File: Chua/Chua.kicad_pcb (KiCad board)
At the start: 2 copper layers, 60 x 30 mm, 19 parts, among them P1 CONN_01X03, U1 TL082, U2 TL082

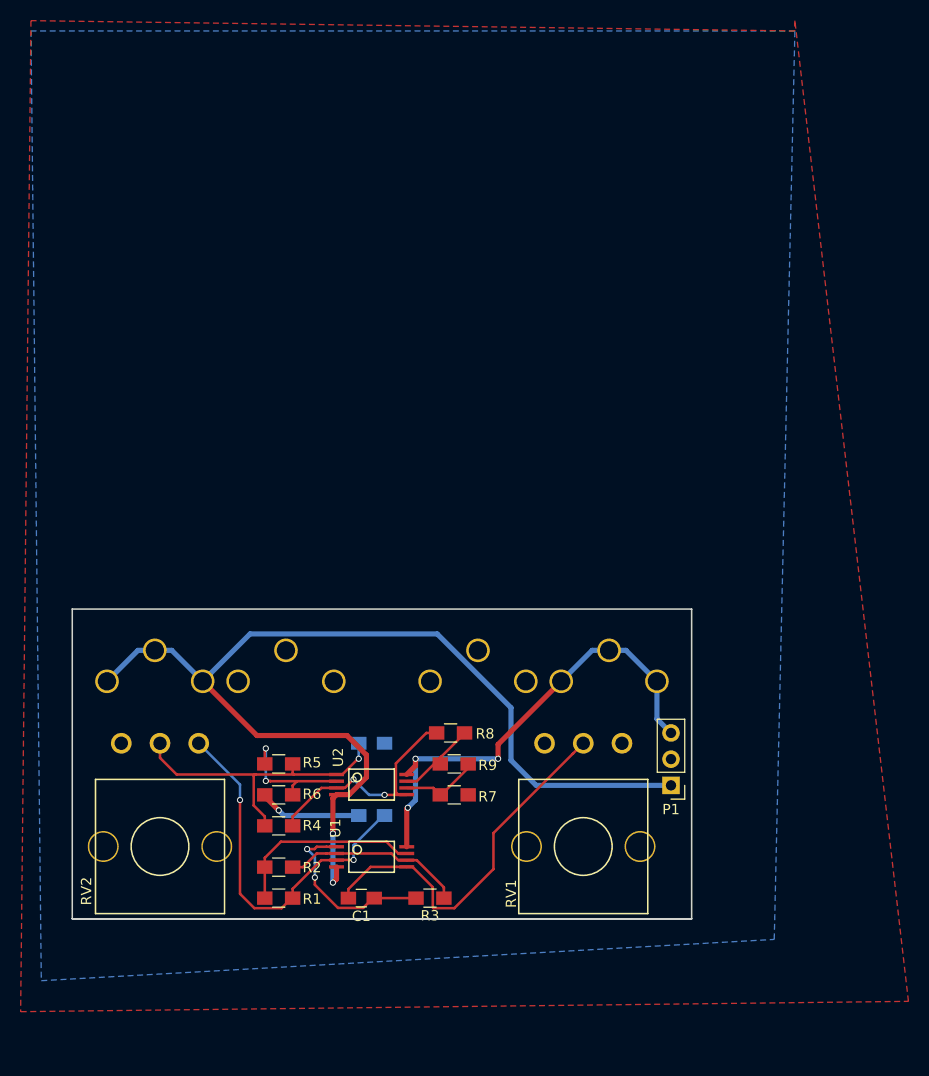
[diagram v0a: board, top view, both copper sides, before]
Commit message: adding output to chua
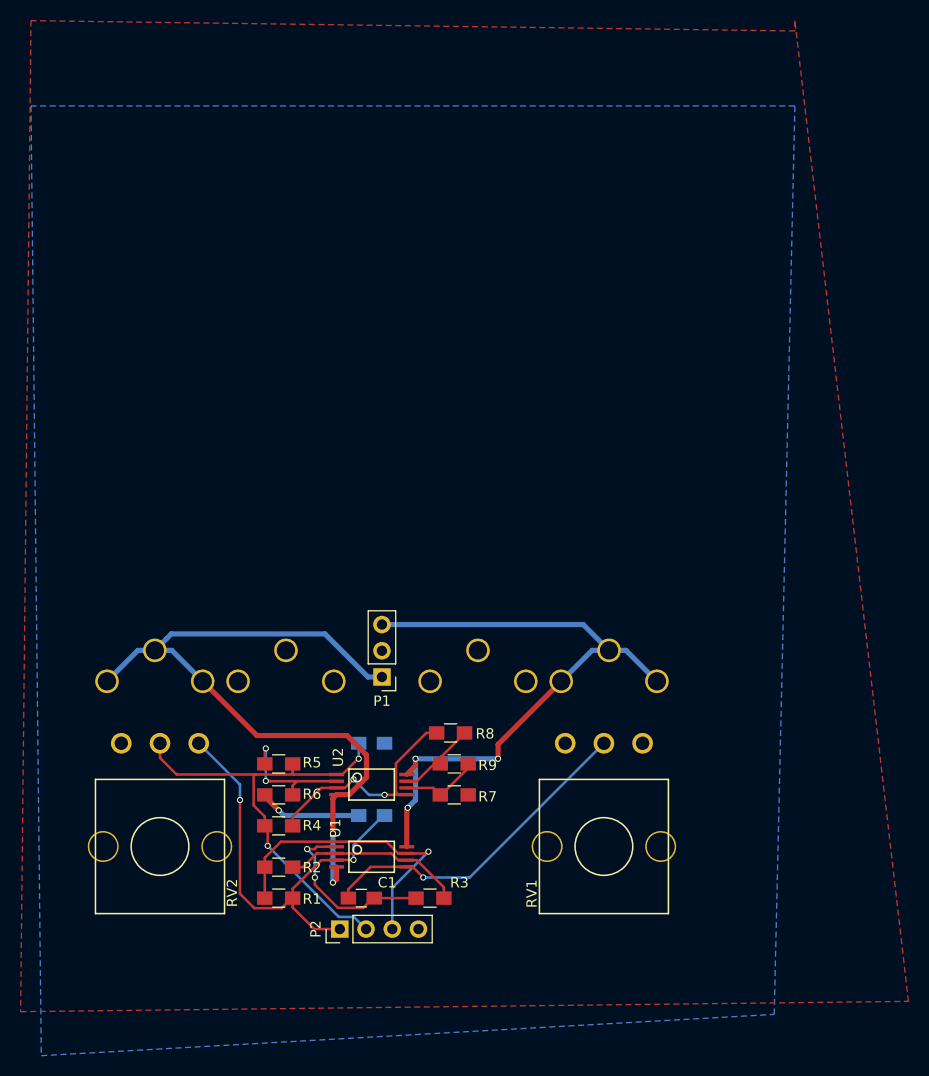
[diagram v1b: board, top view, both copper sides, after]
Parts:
- added P2: CONN_01X04, Pin_Headers:Pin_Header_Straight_1x04_Pitch2.54mm, F.Cu at (95.9, 151.0)
- moved P1 29.9 mm to (100.0, 126.6)
- moved RV1 2.00 mm to (121.5, 143.0)
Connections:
- net Net-(C2-Pad1) renamed /X
- net Net-(C3-Pad1) renamed /Y
- net Net-(R1-Pad2) renamed /P
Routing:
- net /VCC-: track 103.0 -> 71.1 mm
- net /VCC+: track 46.1 -> 63.6 mm
- net /Y: track 30.1 -> 45.0 mm, vias 1 -> 2
- net /P: track 18.8 -> 29.9 mm, vias 0 -> 1
- net /X: track 35.9 -> 42.2 mm
- net Net-(C1-Pad2): track 36.0 -> 32.9 mm, vias 0 -> 1
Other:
- board outline removed
